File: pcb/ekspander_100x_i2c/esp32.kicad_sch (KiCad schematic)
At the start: 7 parts, among them IC1 ESP32-S3-WROOM-1U-N16R8, U13 AP63203WU

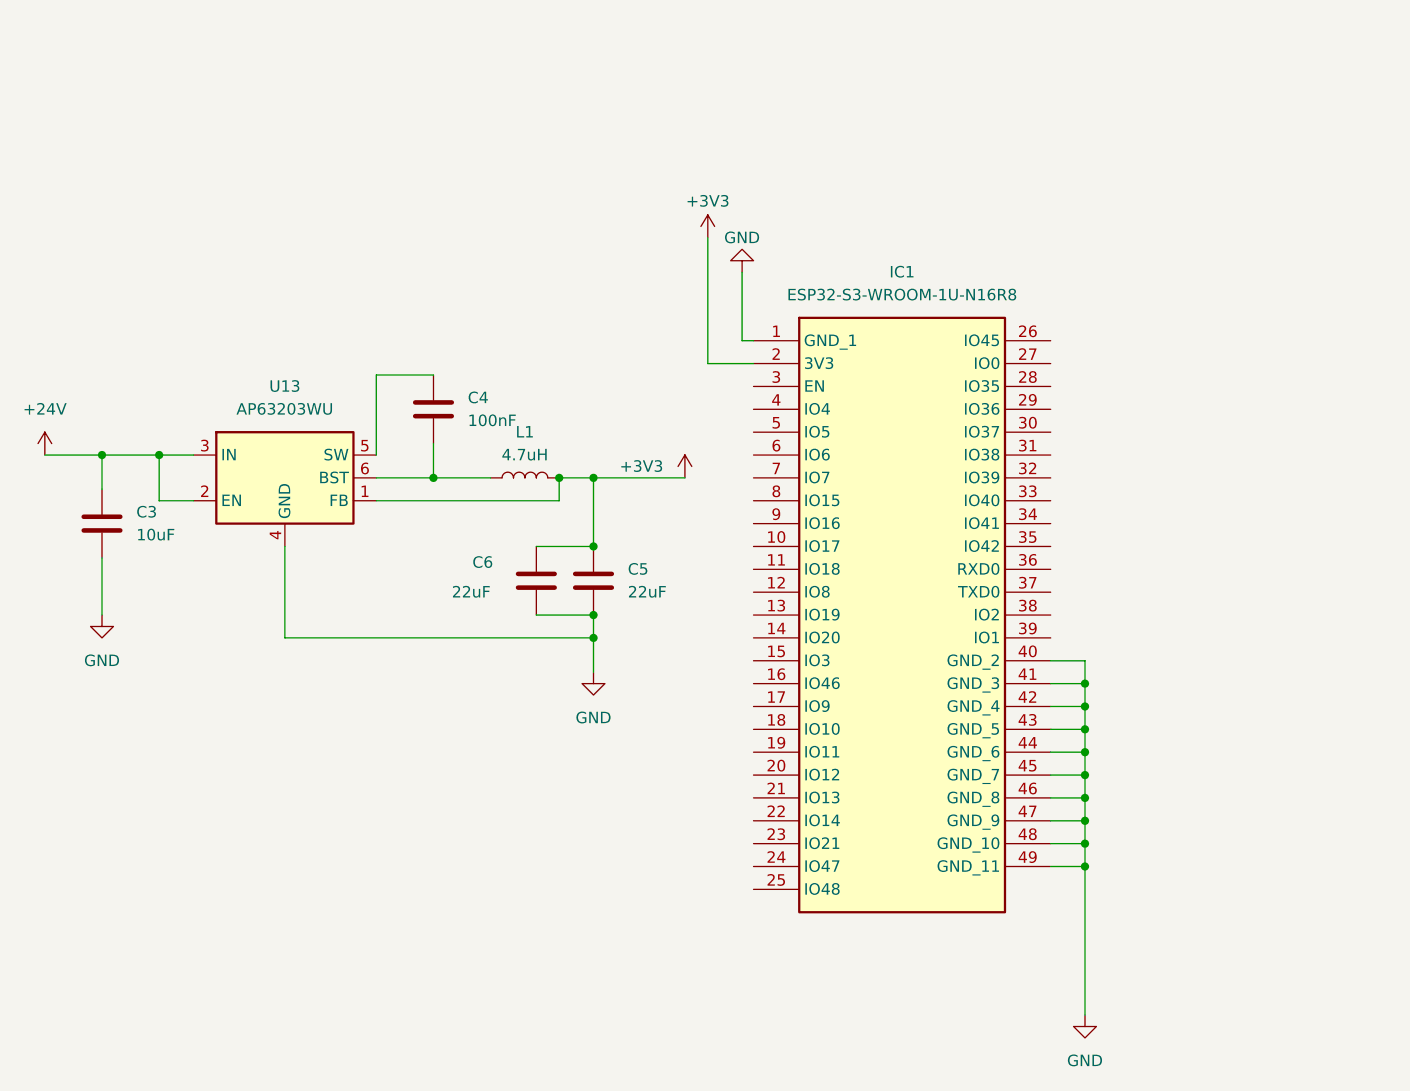
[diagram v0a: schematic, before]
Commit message: Ekspander 100x - zasilanie 3V3
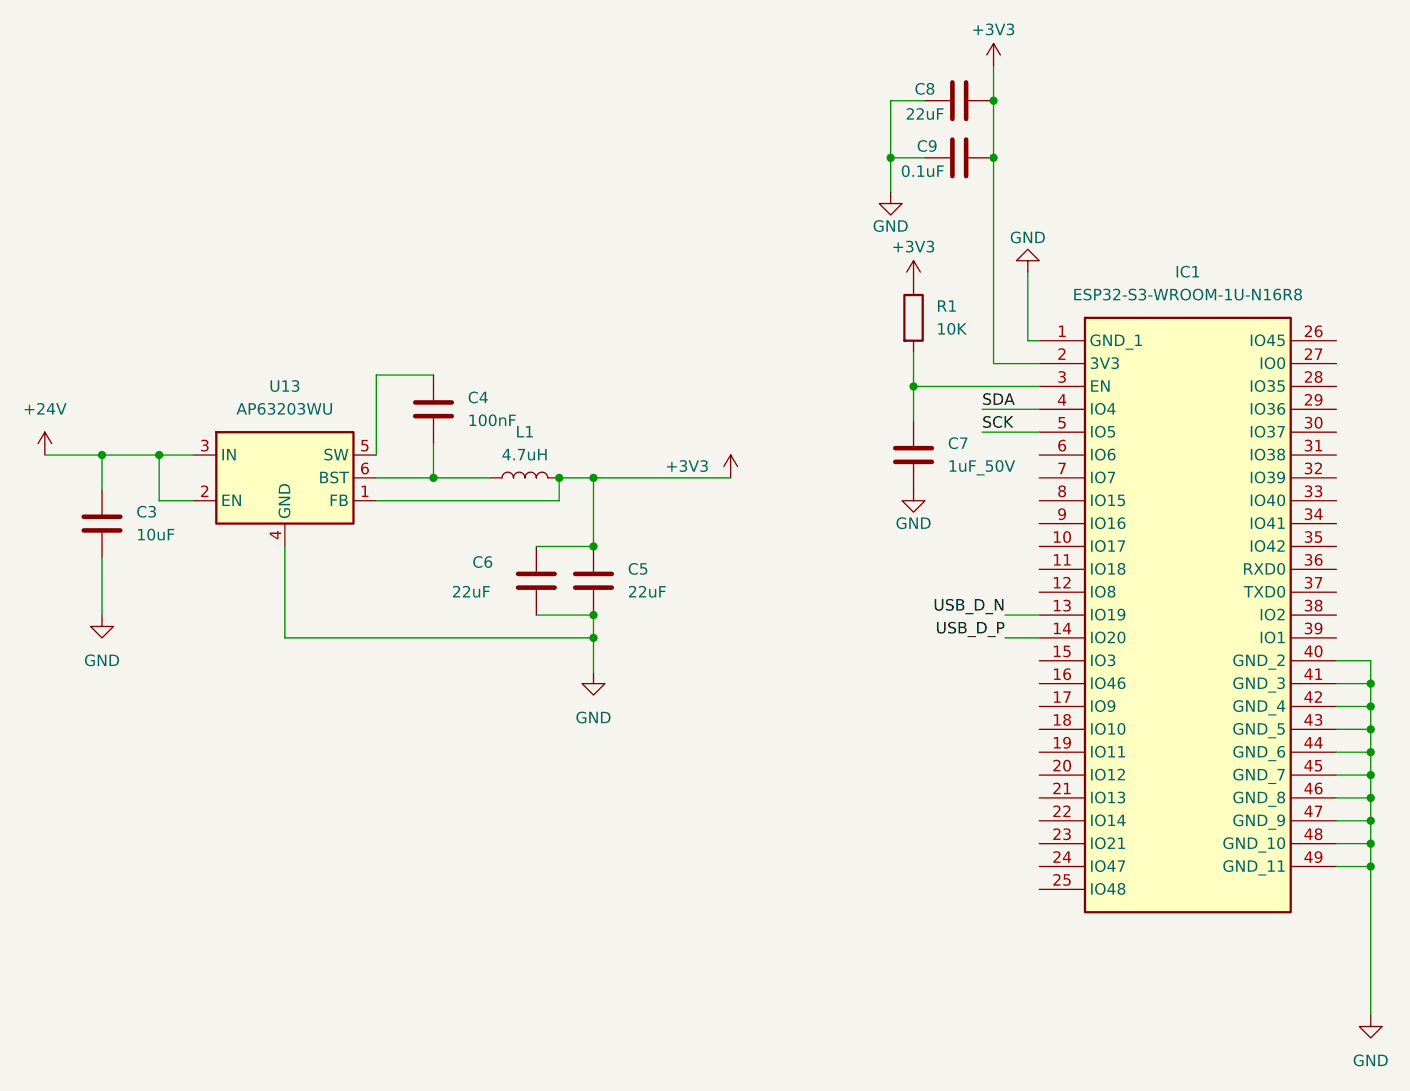
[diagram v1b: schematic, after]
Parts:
- added C7: 1uF_50V, Capacitor_THT:C_Disc_D5.0mm_W2.5mm_P5.00mm, symbol Device:C
- added C8: 22uF, 1_tme:RDEC71H226MWK1H03B, symbol Device:C
- added C9: 0.1uF, 1_tme:RDEC71H226MWK1H03B, symbol Device:C
- added R1: 10K, 1_tme:RESAD1520W50L600D230, symbol Device:R
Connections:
- net +3V3: now also C8.2, C9.2, R1.1
- net GND: now also C7.2, C8.1, C9.1
- net USB_D_N: now reaches IC1.13 (IO19)
- net USB_D_P: now reaches IC1.14 (IO20)
- net at IC1.3 (EN): now also C7.1, R1.2
- net SDA: now reaches IC1.4 (IO4)
- net SCK: now reaches IC1.5 (IO5)
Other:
- moved on the sheet: IC1
